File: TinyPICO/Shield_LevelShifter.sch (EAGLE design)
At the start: 15 parts, among them U4 SN74HCT245DBRDB20-M

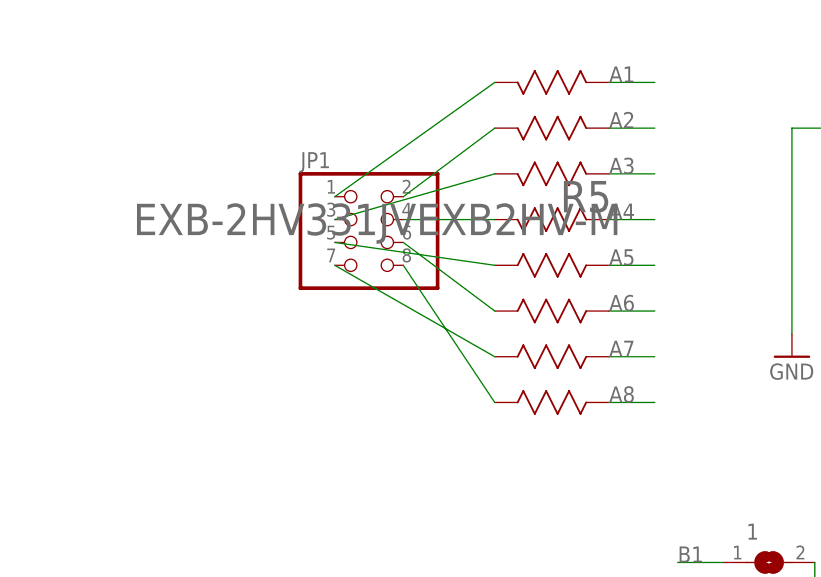
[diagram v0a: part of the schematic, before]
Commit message: Fixing some ERC/DRC errors
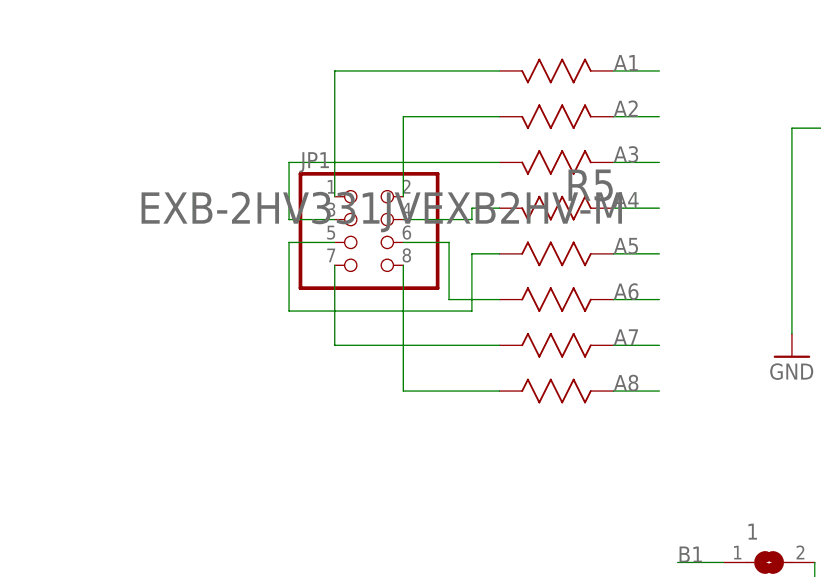
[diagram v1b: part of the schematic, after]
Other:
- moved on the sheet: R5
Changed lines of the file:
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@@
 <attribute name="VALUE" x="99.06" y="124.46" size="1.778" layer="96"/>
 </instance>
-<instance part="R5" gate="A" x="81.28" y="157.48" smashed="yes" rot="MR0">
-<attribute name="VALUE" x="82.6262" y="140.5128" size="3.4798" layer="96" ratio="10" rot="SMR0"/>
-<attribute name="NAME" x="81.5594" y="143.0528" size="3.4798" layer="95" ratio="10" rot="SMR0"/>
+<instance part="R5" gate="A" x="81.788" y="158.75" smashed="yes" rot="MR0">
+<attribute name="VALUE" x="83.1342" y="141.7828" size="3.4798" layer="96" ratio="10" rot="SMR0"/>
+<attribute name="NAME" x="82.0674" y="144.3228" size="3.4798" layer="95" ratio="10" rot="SMR0"/>
 </instance>
 <instance part="3" gate="-0R" x="139.7" y="104.14" smashed="yes" rot="R180">
@@
 </segment>
 </net>
-<net name="N$21" class="0">
-<segment>
-<pinref part="R5" gate="A" pin="16"/>
-<pinref part="JP1" gate="A" pin="1"/>
-<wire x1="68.58" y1="157.48" x2="50.8" y2="144.78" width="0.1524" layer="91"/>
-</segment>
-</net>
-<net name="N$22" class="0">
-<segment>
-<pinref part="R5" gate="A" pin="15"/>
-<pinref part="JP1" gate="A" pin="2"/>
-<wire x1="68.58" y1="152.4" x2="58.42" y2="144.78" width="0.1524" layer="91"/>
-</segment>
-</net>
-<net name="N$23" class="0">
-<segment>
-<pinref part="R5" gate="A" pin="14"/>
-<pinref part="JP1" gate="A" pin="3"/>
-<wire x1="68.58" y1="147.32" x2="50.8" y2="142.24" width="0.1524" layer="91"/>
-</segment>
-</net>
-<net name="N$24" class="0">
-<segment>
-<pinref part="R5" gate="A" pin="13"/>
-<pinref part="JP1" gate="A" pin="4"/>
-<wire x1="68.58" y1="142.24" x2="58.42" y2="142.24" width="0.1524" layer="91"/>
-</segment>
-</net>
-<net name="N$25" class="0">
-<segment>
-<pinref part="R5" gate="A" pin="12"/>
-<pinref part="JP1" gate="A" pin="5"/>
-<wire x1="68.58" y1="137.16" x2="50.8" y2="139.7" width="0.1524" layer="91"/>
-</segment>
-</net>
-<net name="N$26" class="0">
-<segment>
-<pinref part="R5" gate="A" pin="11"/>
-<pinref part="JP1" gate="A" pin="6"/>
-<wire x1="68.58" y1="132.08" x2="58.42" y2="139.7" width="0.1524" layer="91"/>
-</segment>
-</net>
-<net name="N$27" class="0">
-<segment>
-<pinref part="R5" gate="A" pin="10"/>
-<pinref part="JP1" gate="A" pin="7"/>
-<wire x1="68.58" y1="127" x2="50.8" y2="137.16" width="0.1524" layer="91"/>
-</segment>
-</net>
-<net name="N$28" class="0">
-<segment>
-<pinref part="R5" gate="A" pin="9"/>
-<pinref part="JP1" gate="A" pin="8"/>
-<wire x1="68.58" y1="121.92" x2="58.42" y2="137.16" width="0.1524" layer="91"/>
-</segment>
-</net>
 <net name="B1" class="0">
 <segment>
@@
 <segment>
 <pinref part="R5" gate="A" pin="1"/>
-<wire x1="81.28" y1="157.48" x2="86.36" y2="157.48" width="0.1524" layer="91"/>
-<label x="81.28" y="157.48" size="1.778" layer="95"/>
+<wire x1="81.788" y1="158.75" x2="86.868" y2="158.75" width="0.1524" layer="91"/>
+<label x="81.788" y="158.75" size="1.778" layer="95"/>
 </segment>
 </net>
@@
 <segment>
 <pinref part="R5" gate="A" pin="2"/>
-<wire x1="81.28" y1="152.4" x2="86.36" y2="152.4" width="0.1524" layer="91"/>
-<label x="81.28" y="152.4" size="1.778" layer="95"/>
+<wire x1="81.788" y1="153.67" x2="86.868" y2="153.67" width="0.1524" layer="91"/>
+<label x="81.788" y="153.67" size="1.778" layer="95"/>
 </segment>
 </net>
@@
 <segment>
 <pinref part="R5" gate="A" pin="3"/>
-<wire x1="81.28" y1="147.32" x2="86.36" y2="147.32" width="0.1524" layer="91"/>
-<label x="81.28" y="147.32" size="1.778" layer="95"/>
+<wire x1="81.788" y1="148.59" x2="86.868" y2="148.59" width="0.1524" layer="91"/>
+<label x="81.788" y="148.59" size="1.778" layer="95"/>
 </segment>
 </net>
@@
 <segment>
 <pinref part="R5" gate="A" pin="4"/>
-<wire x1="81.28" y1="142.24" x2="86.36" y2="142.24" width="0.1524" layer="91"/>
-<label x="81.28" y="142.24" size="1.778" layer="95"/>
+<wire x1="81.788" y1="143.51" x2="86.868" y2="143.51" width="0.1524" layer="91"/>
+<label x="81.788" y="143.51" size="1.778" layer="95"/>
 </segment>
 </net>
@@
 <segment>
 <pinref part="R5" gate="A" pin="5"/>
-<wire x1="81.28" y1="137.16" x2="86.36" y2="137.16" width="0.1524" layer="91"/>
-<label x="81.28" y="137.16" size="1.778" layer="95"/>
+<wire x1="81.788" y1="138.43" x2="86.868" y2="138.43" width="0.1524" layer="91"/>
+<label x="81.788" y="138.43" size="1.778" layer="95"/>
 </segment>
 </net>
@@
 <segment>
 <pinref part="R5" gate="A" pin="6"/>
-<wire x1="81.28" y1="132.08" x2="86.36" y2="132.08" width="0.1524" layer="91"/>
-<label x="81.28" y="132.08" size="1.778" layer="95"/>
+<wire x1="81.788" y1="133.35" x2="86.868" y2="133.35" width="0.1524" layer="91"/>
+<label x="81.788" y="133.35" size="1.778" layer="95"/>
 </segment>
 </net>
@@
 <segment>
 <pinref part="R5" gate="A" pin="7"/>
-<wire x1="81.28" y1="127" x2="86.36" y2="127" width="0.1524" layer="91"/>
-<label x="81.28" y="127" size="1.778" layer="95"/>
+<wire x1="81.788" y1="128.27" x2="86.868" y2="128.27" width="0.1524" layer="91"/>
+<label x="81.788" y="128.27" size="1.778" layer="95"/>
 </segment>
 </net>
@@
 <segment>
 <pinref part="R5" gate="A" pin="8"/>
-<wire x1="81.28" y1="121.92" x2="86.36" y2="121.92" width="0.1524" layer="91"/>
-<label x="81.28" y="121.92" size="1.778" layer="95"/>
-</segment>
-</net>
+<wire x1="81.788" y1="123.19" x2="86.868" y2="123.19" width="0.1524" layer="91"/>
+<label x="81.788" y="123.19" size="1.778" layer="95"/>
+</segment>
+</net>
+<net name="N$1" class="0">
+<segment>
+<pinref part="JP1" gate="A" pin="1"/>
+<pinref part="R5" gate="A" pin="16"/>
+<wire x1="69.088" y1="158.75" x2="50.8" y2="158.75" width="0.1524" layer="91"/>
+<wire x1="50.8" y1="158.75" x2="50.8" y2="144.78" width="0.1524" layer="91"/>
+</segment>
+</net>
+<net name="N$3" class="0">
+<segment>
+<pinref part="R5" gate="A" pin="15"/>
+<wire x1="69.088" y1="153.67" x2="58.42" y2="153.67" width="0.1524" layer="91"/>
+<pinref part="JP1" gate="A" pin="2"/>
+<wire x1="58.42" y1="153.67" x2="58.42" y2="144.78" width="0.1524" layer="91"/>
+</segment>
+</net>
+<net name="N$4" class="0">
+<segment>
+<pinref part="R5" gate="A" pin="14"/>
+<wire x1="69.088" y1="148.59" x2="45.72" y2="148.59" width="0.1524" layer="91"/>
+<wire x1="45.72" y1="148.59" x2="45.72" y2="142.24" width="0.1524" layer="91"/>
+<pinref part="JP1" gate="A" pin="3"/>
+<wire x1="45.72" y1="142.24" x2="50.8" y2="142.24" width="0.1524" layer="91"/>
+</segment>
+</net>
+<net name="N$2" class="0">
+<segment>
+<pinref part="R5" gate="A" pin="13"/>
+<wire x1="69.088" y1="143.51" x2="66.04" y2="143.51" width="0.1524" layer="91"/>
+<wire x1="66.04" y1="143.51" x2="66.04" y2="142.24" width="0.1524" layer="91"/>
+<pinref part="JP1" gate="A" pin="4"/>
+<wire x1="66.04" y1="142.24" x2="58.42" y2="142.24" width="0.1524" layer="91"/>
+</segment>
+</net>
+<net name="N$5" class="0">
+<segment>
+<pinref part="R5" gate="A" pin="12"/>
+<wire x1="69.088" y1="138.43" x2="66.04" y2="138.43" width="0.1524" layer="91"/>
+<wire x1="66.04" y1="138.43" x2="66.04" y2="132.08" width="0.1524" layer="91"/>
+<wire x1="66.04" y1="132.08" x2="45.72" y2="132.08" width="0.1524" layer="91"/>
+<wire x1="45.72" y1="132.08" x2="45.72" y2="139.7" width="0.1524" layer="91"/>
+<pinref part="JP1" gate="A" pin="5"/>
+<wire x1="45.72" y1="139.7" x2="50.8" y2="139.7" width="0.1524" layer="91"/>
+</segment>
+</net>
+<net name="N$6" class="0">
+<segment>
+<pinref part="R5" gate="A" pin="11"/>
+<wire x1="69.088" y1="133.35" x2="63.5" y2="133.35" width="0.1524" layer="91"/>
+<wire x1="63.5" y1="133.35" x2="63.5" y2="139.7" width="0.1524" layer="91"/>
+<pinref part="JP1" gate="A" pin="6"/>
+<wire x1="63.5" y1="139.7" x2="58.42" y2="139.7" width="0.1524" layer="91"/>
+</segment>
+</net>
+<net name="N$7" class="0">
+<segment>
+<pinref part="R5" gate="A" pin="10"/>
+<wire x1="69.088" y1="128.27" x2="50.8" y2="128.27" width="0.1524" layer="91"/>
+<wire x1="50.8" y1="128.27" x2="50.8" y2="137.16" width="0.1524" layer="91"/>
+<pinref part="JP1" gate="A" pin="7"/>
+</segment>
+</net>
+<net name="N$8" class="0">
+<segment>
+<pinref part="R5" gate="A" pin="9"/>
+<wire x1="69.088" y1="123.19" x2="58.42" y2="123.19" width="0.1524" layer="91"/>
+<pinref part="JP1" gate="A" pin="8"/>
+<wire x1="58.42" y1="123.19" x2="58.42" y2="137.16" width="0.1524" layer="91"/>
+</segment>
+</net>
